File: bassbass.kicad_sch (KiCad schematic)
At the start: 42 parts, among them P1 USB_C_Plug_USB2.0, Q1 Q_NPN_BEC, SW1 SW_SPDT, SW2 SW_SPDT, U1 4069, U2 TLV61048

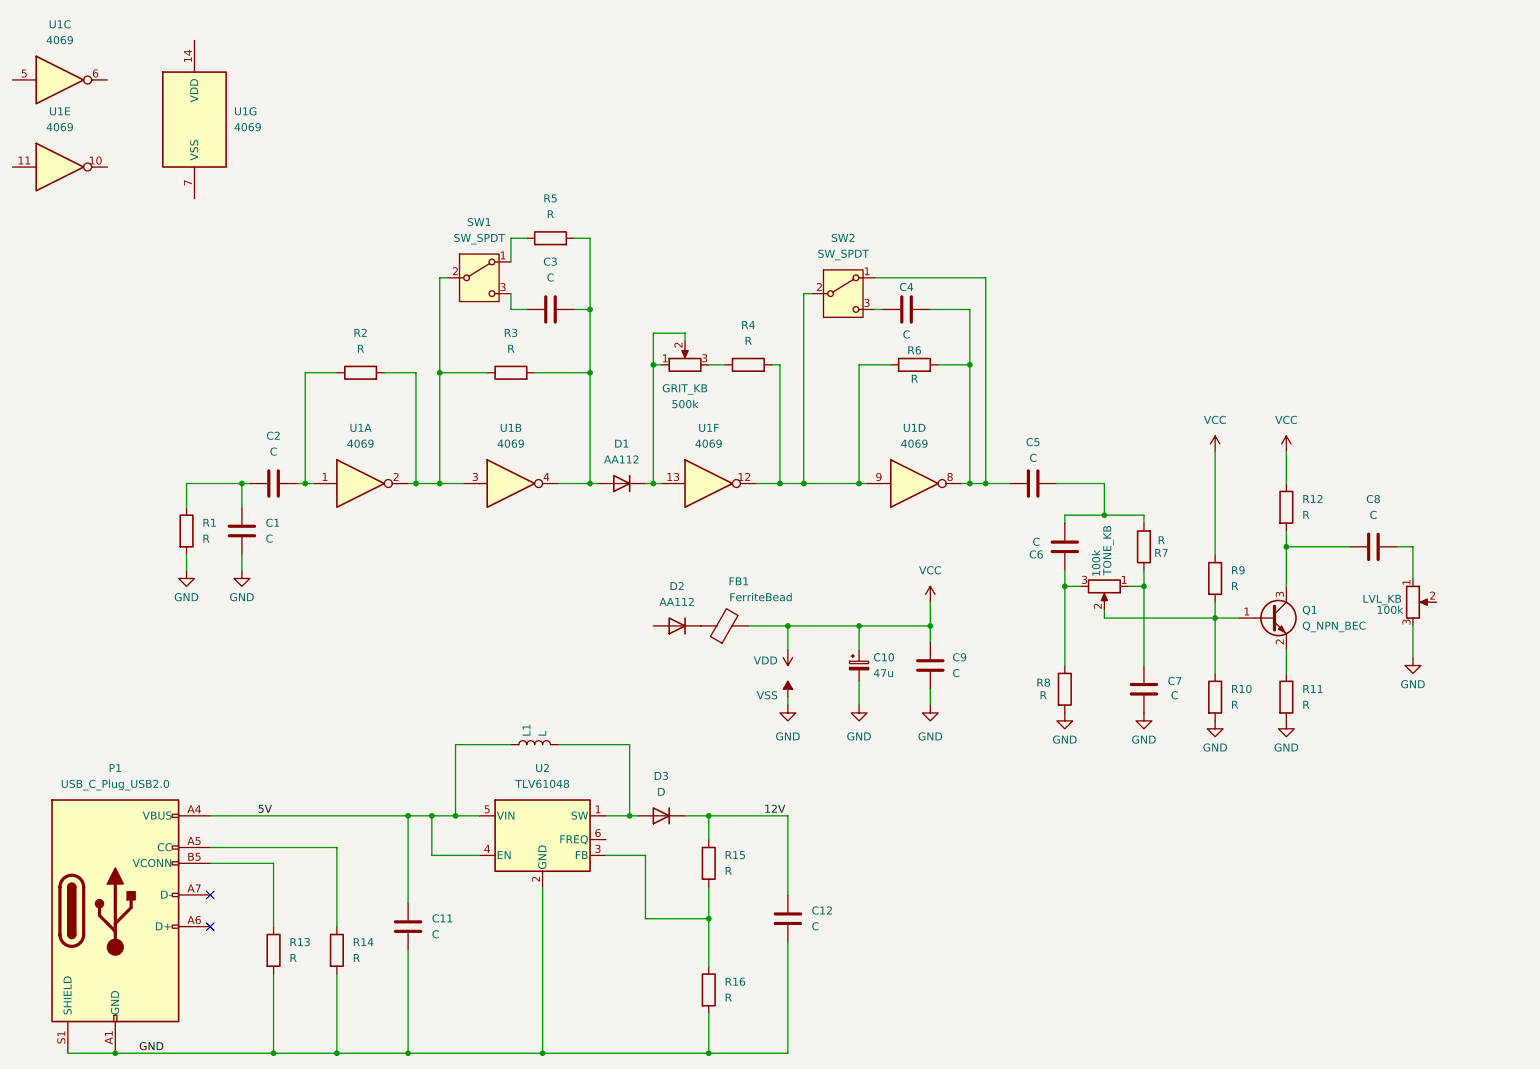
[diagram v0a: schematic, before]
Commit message: progress
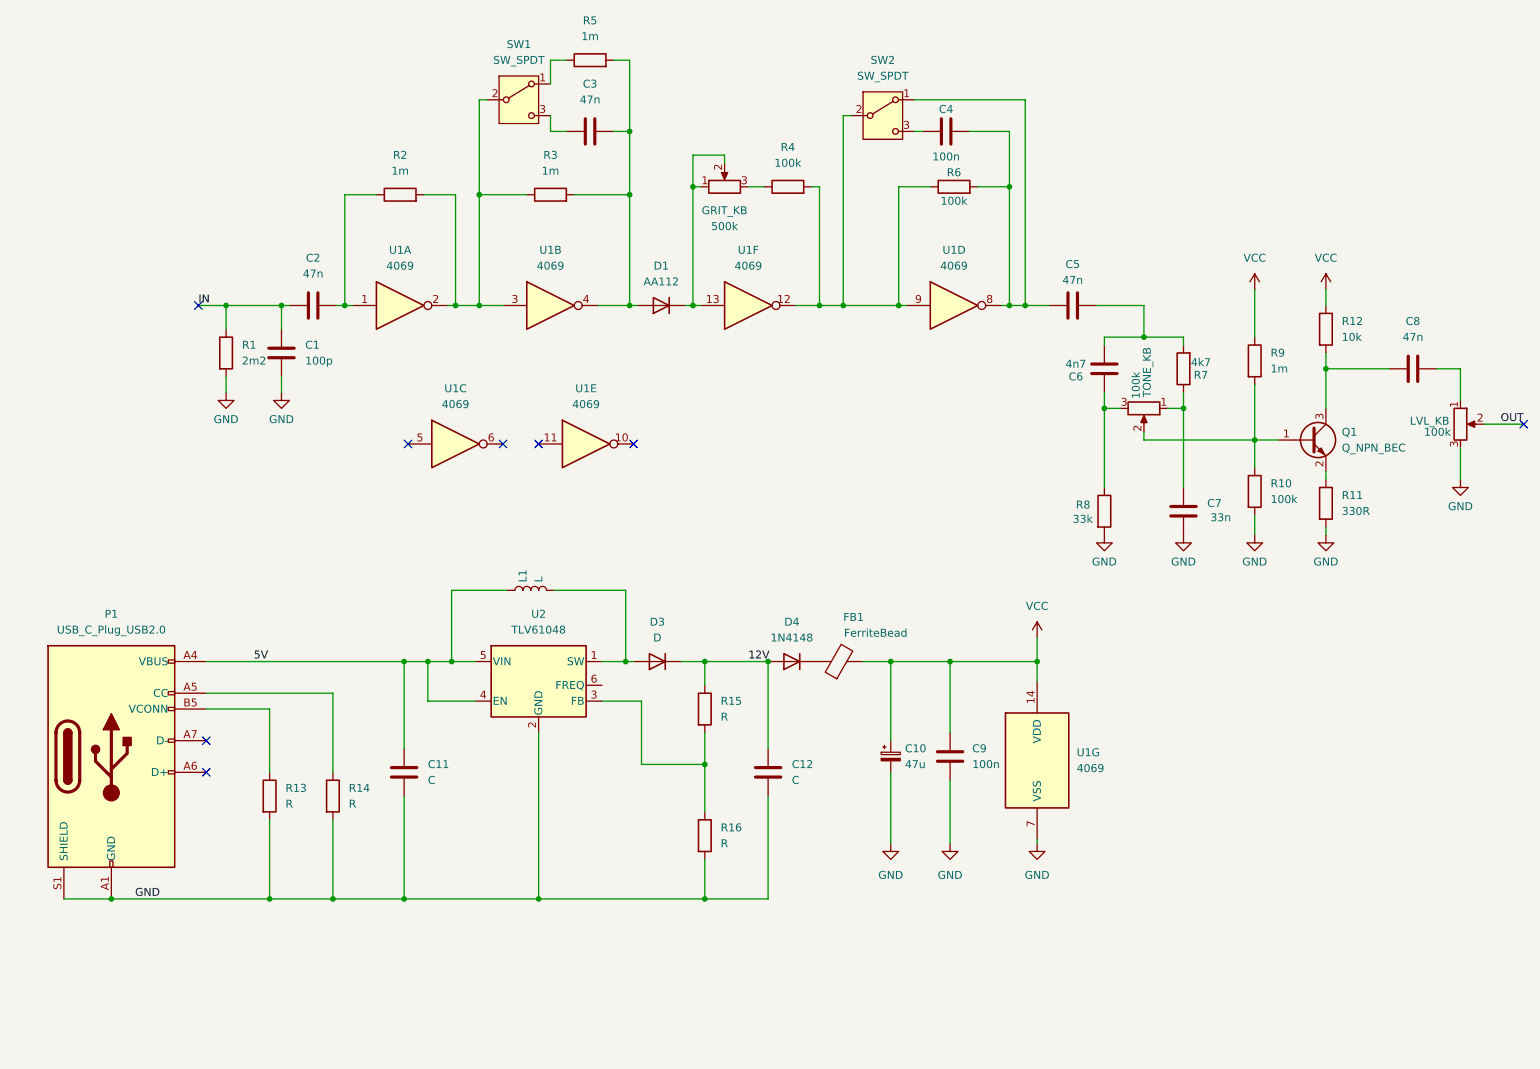
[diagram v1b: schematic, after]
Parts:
- removed D2: AA112, Diode_SMD:D_SOD-123, symbol Diode:BAV16W
- added D4: 1N4148, Diode_THT:D_DO-35_SOD27_P7.62mm_Horizontal, symbol Diode:1N4148
- C1: value C -> 100p
- C2, C3, C5, C8: value C -> 47n
- C4, C9: value C -> 100n
- C6: value C -> 4n7
- C7: value C -> 33n
- R1: value R -> 2m2
- R10, R4, R6: value R -> 100k
- R11: value R -> 330R
- R12: value R -> 10k
- R2, R3, R5, R9: value R -> 1m
- R7: value R -> 4k7
- R8: value R -> 33k
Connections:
- net 12V: now also D4.2 (A)
- net GND: now also U1.7 (VSS)
- net VCC: now also U1.14 (VDD)
- net IN: now reaches C1.1, C2.1, R1.1
- net at FB1.1: now also D4.1 (K)
- net OUT: now reaches LVL_KB.2
- no-connect marks 2 -> 8
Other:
- moved on the sheet: C1, C10, C11, C12, C2, C3, C4, C5, C6, C7, C8, C9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
